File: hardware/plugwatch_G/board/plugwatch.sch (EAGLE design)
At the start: 113 parts, among them J1 DM3AT-SF-PEJM5, J2 SCREW_TERMNIAL_1, J3 SCREW_TERMNIAL_1, Q1 NX3008PBK, Q2 MOSFET-NCHANNELSMD, U1 AB1815-T3, U10 OPA369, U11 SIP32510, U12 SIP32510, U14 SIP32510, U2 BGA725L6-ALT, U3 DS2401P+, U4 SAFFB1G56KB0F0A, U5 IRM-03-5V, U6 LIS2DH12, U7 MAX-M8, U8 MAX67XXMAX6749MAX67XX, U9 OPA369, X1 ABS07-32.768KHZ-7-T

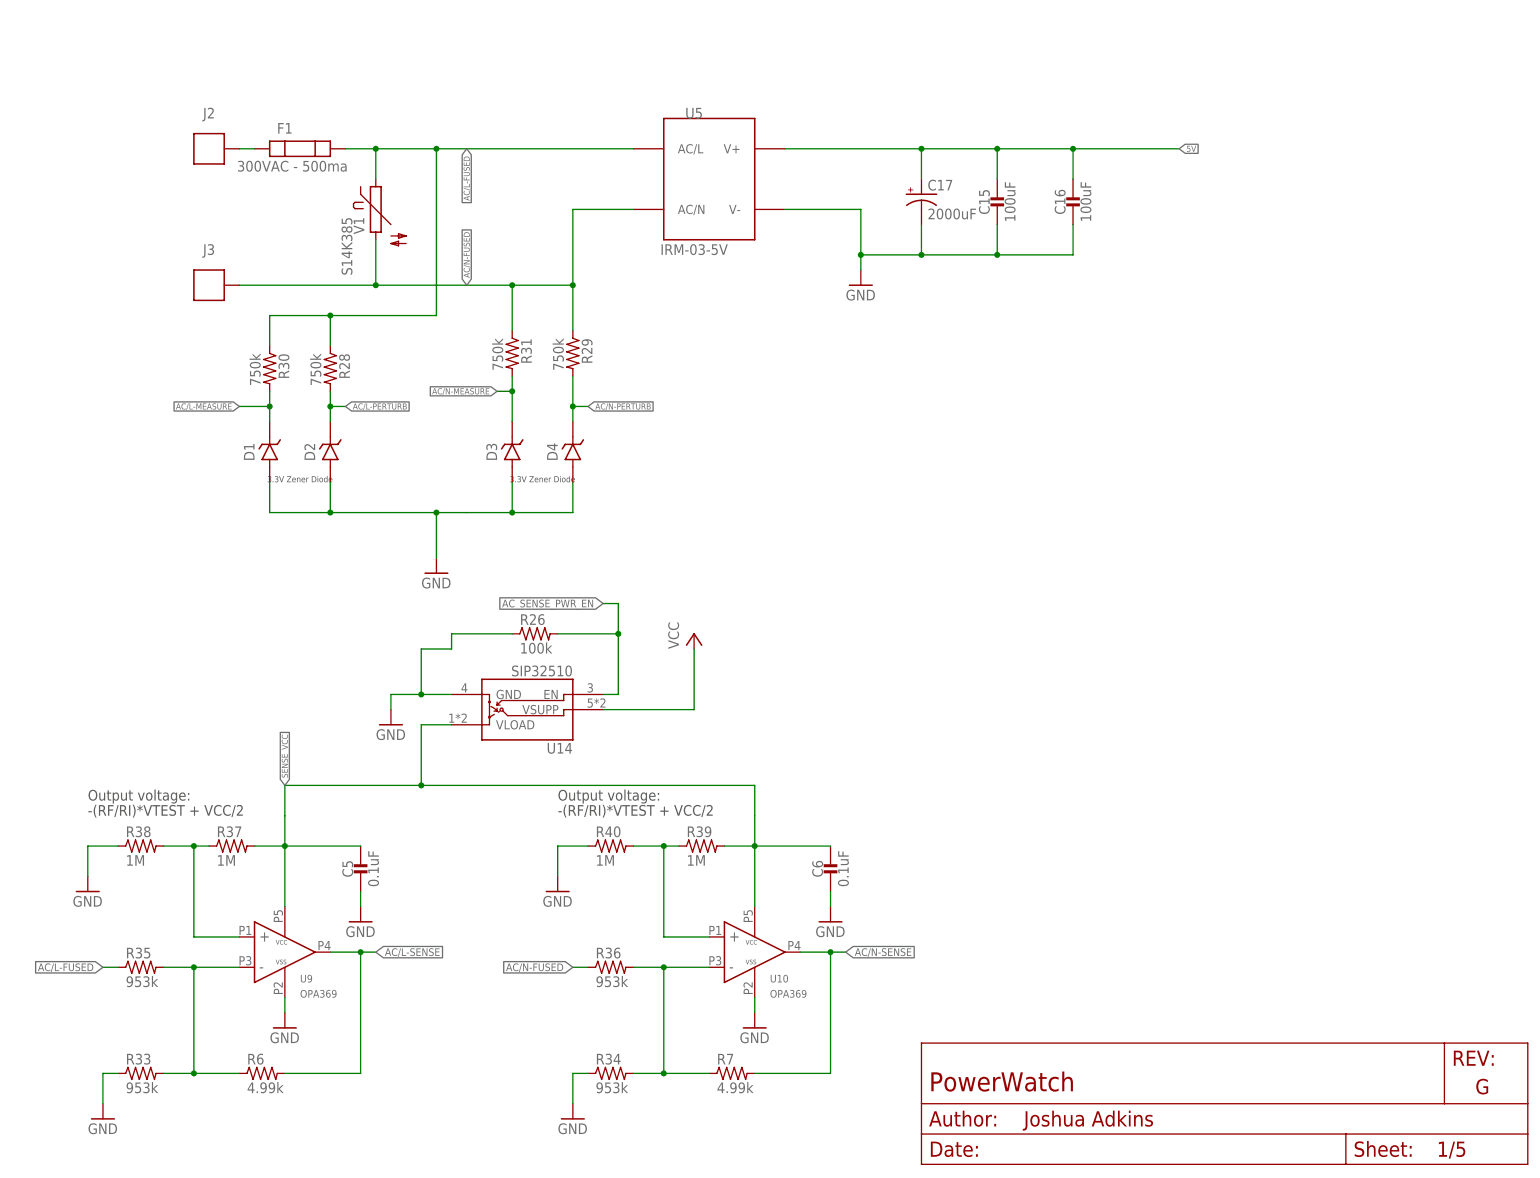
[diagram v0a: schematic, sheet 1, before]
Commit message: add new voltage amplifier circuit
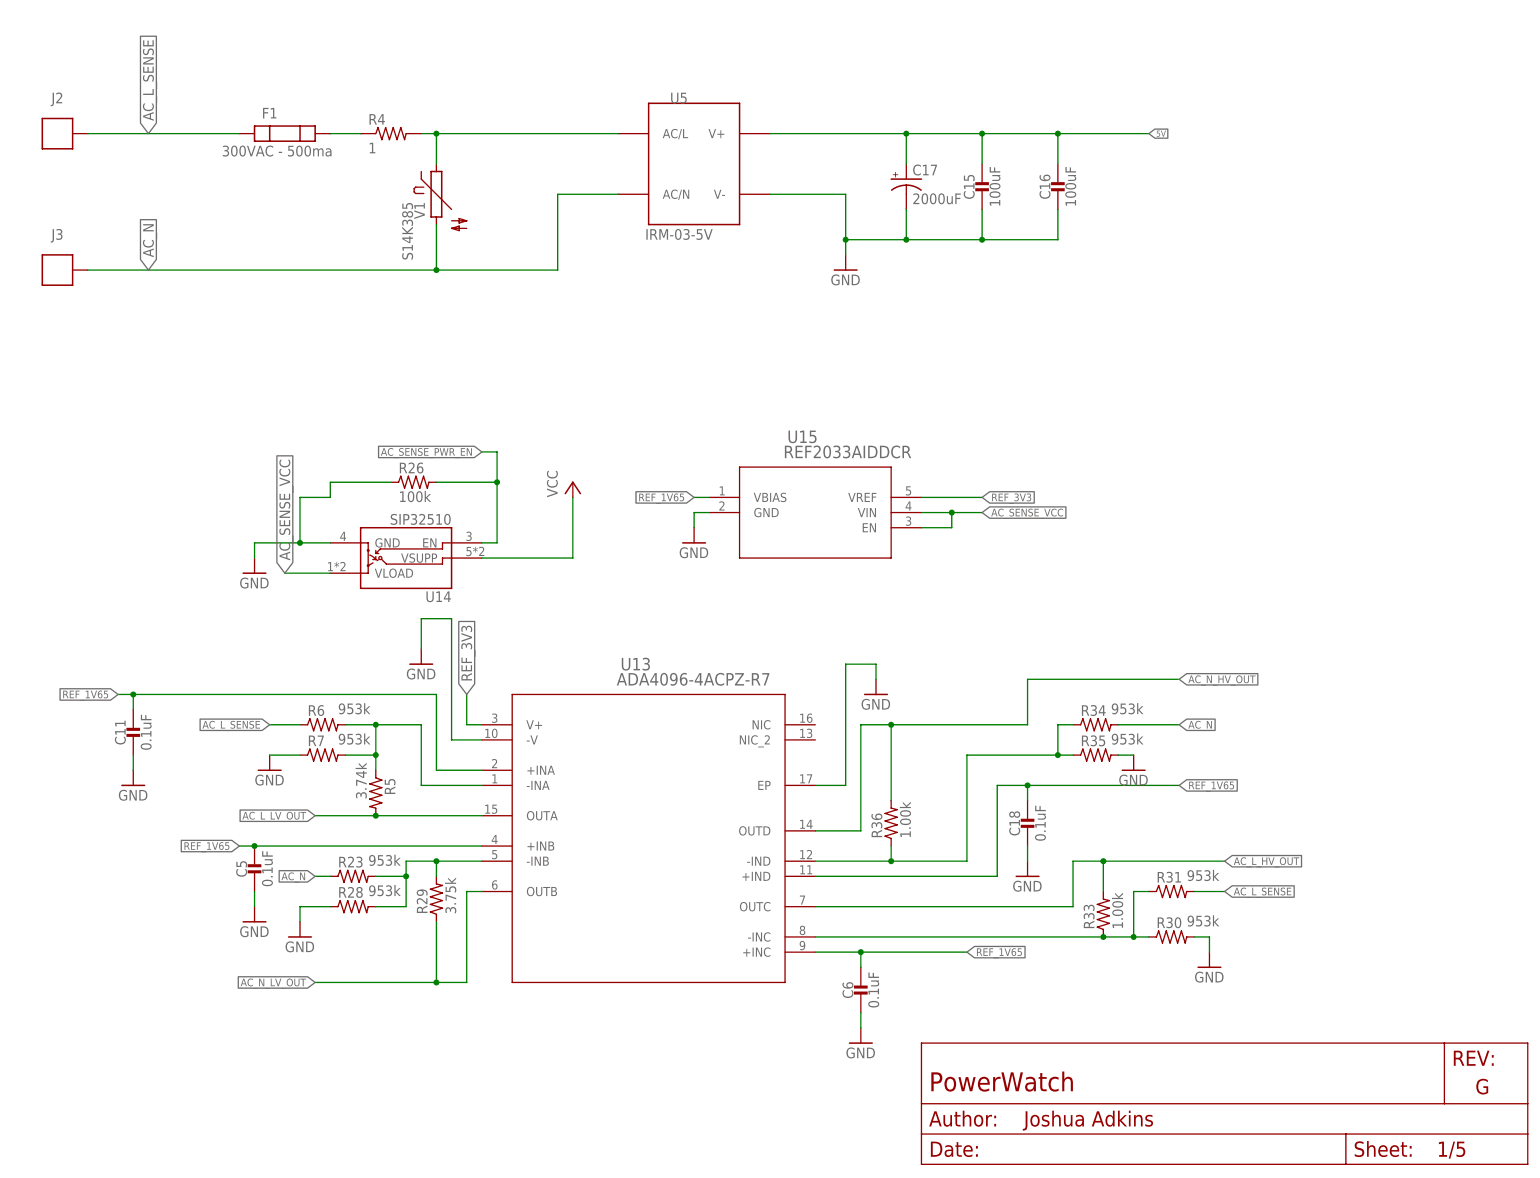
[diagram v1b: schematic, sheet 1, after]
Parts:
- removed D1, D2, D3, D4: (no value), passives:DIODE_ZENERSOT323
- removed R37, R38, R39, R40: 1M, passives:RESISTOR0402_RES
- removed U10, U9: OPA369, powerfilm:OPA369
- added C11, C18: 0.1uF, passives:CAPACITOR0402_CAP
- added R23: 953k, passives:RESISTOR0402_RES
- added R4: 1, resistor:R-US_R2512
- added R5: 3.74k, passives:RESISTOR0402_RES
- added U13: ADA4096-4ACPZ-R7, ada4096-4:ADA4096-4ACPZ-R7
- added U15: REF2033AIDDCR, ref2033:REF2033AIDDCR
- R28, R30, R31: value 750k -> 953k; device passives:RESISTOR1206_RES_HIGH_CLEARANCE -> passives:RESISTOR0402_RES; DESCRIPTION RES SMD 750K OHM 1% 1/4W 1206 -> RES SMD 100K OHM 1% 1/16W 0402; DIGIKEY 311-750KFRCT-ND -> 541-100KLCT-ND; MANUFACTURER Yageo -> Vishay Dale; MPN RC1206FR-07750KL -> CRCW0402100KFKED
- R29: value 750k -> 3.75k; device passives:RESISTOR1206_RES_HIGH_CLEARANCE -> passives:RESISTOR0402_RES; DESCRIPTION RES SMD 750K OHM 1% 1/4W 1206 -> RES SMD 100K OHM 1% 1/16W 0402; DIGIKEY 311-750KFRCT-ND -> 541-100KLCT-ND; MANUFACTURER Yageo -> Vishay Dale; MPN RC1206FR-07750KL -> CRCW0402100KFKED
- R33: value 953k -> 1.00k; DESCRIPTION RES SMD 953K OHM 1% 1/16W 0402 -> RES SMD 100K OHM 1% 1/16W 0402; DIGIKEY YAG3262CT-ND -> 541-100KLCT-ND; MANUFACTURER Yageo -> Vishay Dale; MPN RC0402FR-07953KL -> CRCW0402100KFKED
- R34: DESCRIPTION RES SMD 953K OHM 1% 1/16W 0402 -> RES SMD 100K OHM 1% 1/16W 0402; DIGIKEY YAG3262CT-ND -> 541-100KLCT-ND; MANUFACTURER Yageo -> Vishay Dale; MPN RC0402FR-07953KL -> CRCW0402100KFKED
- R35: device passives:RESISTOR1206_RES_HIGH_CLEARANCE -> passives:RESISTOR0402_RES; DESCRIPTION (none) -> RES SMD 100K OHM 1% 1/16W 0402; DIGIKEY P953KBCCT-ND -> 541-100KLCT-ND; MANUFACTURER Panasonic Electronic Components -> Vishay Dale; MPN ERA-8AEB9533V -> CRCW0402100KFKED
- R36: value 953k -> 1.00k; device passives:RESISTOR1206_RES_HIGH_CLEARANCE -> passives:RESISTOR0402_RES; DESCRIPTION (none) -> RES SMD 100K OHM 1% 1/16W 0402; DIGIKEY P953KBCCT-ND -> 541-100KLCT-ND; MANUFACTURER Panasonic Electronic Components -> Vishay Dale; MPN ERA-8AEB9533V -> CRCW0402100KFKED
- R6, R7: value 4.99k -> 953k; DESCRIPTION RES SMD 4.99K OHM 1% 1/10W 0402 -> RES SMD 100K OHM 1% 1/16W 0402; DIGIKEY P4.99KLCT-ND -> 541-100KLCT-ND; MANUFACTURER Panasonic Electronic Components -> Vishay Dale; MPN ERJ-2RKF4991X -> CRCW0402100KFKED
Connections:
- removed net AC/L-FUSED: F1.P$2, R28.1, R30.1, R35.1, U5.AC/L, V1.1
- removed net AC/N-FUSED: J3.P$1, R29.1, R31.1, R36.1, U5.AC/N, V1.2
- removed net N$38: F1.P$1, J2.P$1
- removed net N$42: R37.1, R38.2, U9.IN+
- removed net N$43: R33.2, R35.2, R6.1, U9.IN-
- removed net N$44: R39.1, R40.2, U10.IN+
- removed net N$45: R34.2, R36.2, R7.1, U10.IN-
- removed net SENSE_VCC: C5.1, C6.1, R37.2, R39.2, U10.VCC, U14.VLOAD, U9.VCC
- new net AC_L_HV_OUT: R33.2, U13.OUTC
- new net AC_L_LV_OUT: R5.2, U13.OUTA
- new net AC_L_SENSE: F1.P$1, J2.P$1, R31.2, R6.1
- new net AC_N: J3.P$1, R23.1, R34.2, U5.AC/N, V1.2
- new net AC_N_HV_OUT: R36.2, U13.OUTD
- new net AC_N_LV_OUT: R29.1, U13.OUTB
- new net AC_SENSE_VCC: U14.VLOAD, U15.EN, U15.VIN
- new net N$1: F1.P$2, R4.1
- new net N$2: R4.2, U5.AC/L, V1.1
- new net N$3: R23.2, R28.2, R29.2, U13.-INB
- new net N$4: R5.1, R6.2, R7.2, U13.-INA
- new net N$6: R30.1, R31.1, R33.1, U13.-INC
- new net N$8: R34.1, R35.1, R36.1, U13.-IND
- new net REF_1V65: C11.1, C18.1, C5.1, C6.1, U13.+INA, U13.+INB, U13.+INC, U13.+IND, U15.VBIAS
- new net REF_3V3: U13.V+, U15.VREF
- net AC/L-MEASURE: no longer D1.CATHODE, R30.2
- net AC/L-PERTURB: no longer D2.CATHODE, R28.2
- net AC/L-SENSE: no longer R6.2, U9.OUT
- net AC/N-MEASURE: no longer D3.CATHODE, R31.2
- net AC/N-PERTURB: no longer D4.CATHODE, R29.2
- net AC/N-SENSE: no longer R7.2, U10.OUT
- net GND: now also C11.2, C18.2, R28.1, R30.2, R35.2, R7.1, U13.-V, U13.EP, U15.GND; no longer D1.ANODE, D2.ANODE, D3.ANODE, D4.ANODE, R33.1, R34.1, R38.1, R40.1, U10.VSS, U9.VSS
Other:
- note added: "There are two goals of the sensing circuit: 1) be able to sense voltages precisely from 0-340vpp and less precisely from 340-1500vpp. 2) Protect the AC/DC converter which has a maximum voltage of 280vac rms. The theory of operation here is that in normal mode the MOV isn't conducting, current through R4 is rather low, and it's power dissipation is also low. In a voltage spike scenario the MOV wil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"
- note added: "This op amp has built in over voltage protection, so while op-amps A and B experience > 3.3V on their input in high voltage scenarios the op amp is made to handle that."
- note added: "This ref supplies 20ma at low (300mv) drop out. We can use it to supply VDDA of the MCU, the Amps and bias the non-inverting side of the amps. Using the same source for all of this should eliminate many sources of noise."
- note removed: "-(RF/RI)*VTEST + VCC/2"
- note removed: "3.3V Zener Diode"
- note removed: "Assuming 340Vpp, a 750k resistor will dissipate 0.15W, and a 3.3v zener will dissipate 1.4mW"
- note removed: "Output voltage:"
- note removed: "The schottkey diode is necessary to protect the MCU pin against the -0.7-1V potentially caused by the zener forward voltage if AC/L or AC/N are negative relative to GND. The schottkey has Vf < 0.3 which is less than the internal diodes on most MCUs."
- note removed: "This circuit handles up to 340V with a 3.3V reference."
- note removed: "We use a seperate AC Measure pin so that we can more directly sense the perturbation by the digital output. The full-scale voltage sensing circuit (below) could also be used, but would only sense <1% of its dynamic range."
- moved on the sheet: C15, C16, C17, C5, C6, F1, J2, J3, R26, R28, R29, R30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
